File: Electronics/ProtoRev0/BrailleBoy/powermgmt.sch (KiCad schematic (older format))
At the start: 13 parts, among them J1 USB_B_Micro, J2 Battery, U4 AP2115-SOIC, U5 MCP73832-2-OT

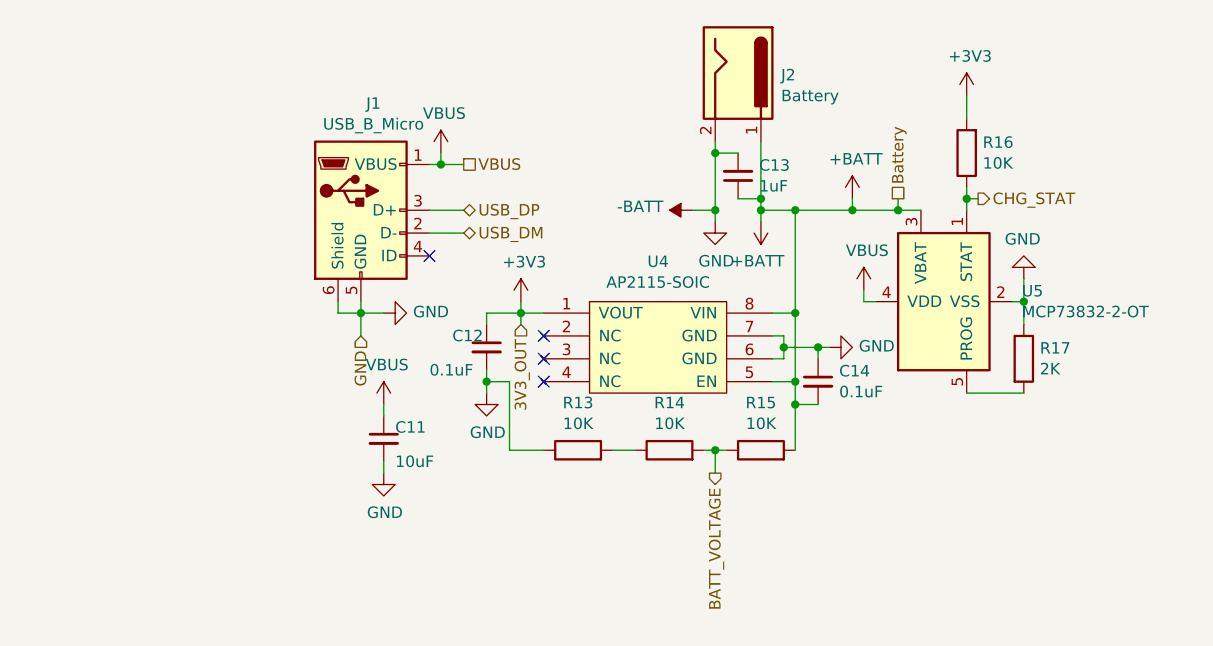
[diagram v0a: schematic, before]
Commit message: Added some annotations to make things rather professional :)
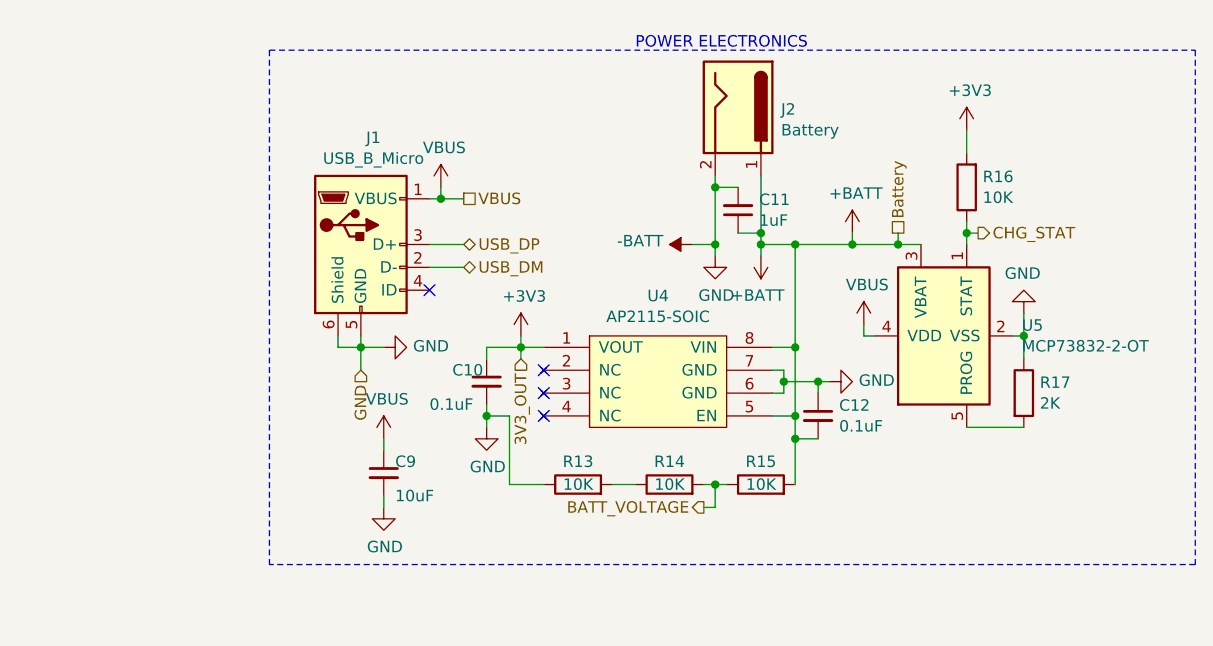
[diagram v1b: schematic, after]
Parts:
- renumbered C12 to C10, C13 to C11, C14 to C12, C11 to C9
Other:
- note added: "POWER ELECTRONICS"
- moved on the sheet: C10, C11, C12, C9, J1, J2, R13, R14, R15, R16, R17, U4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

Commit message: Made the schematic sheets a bit prettier
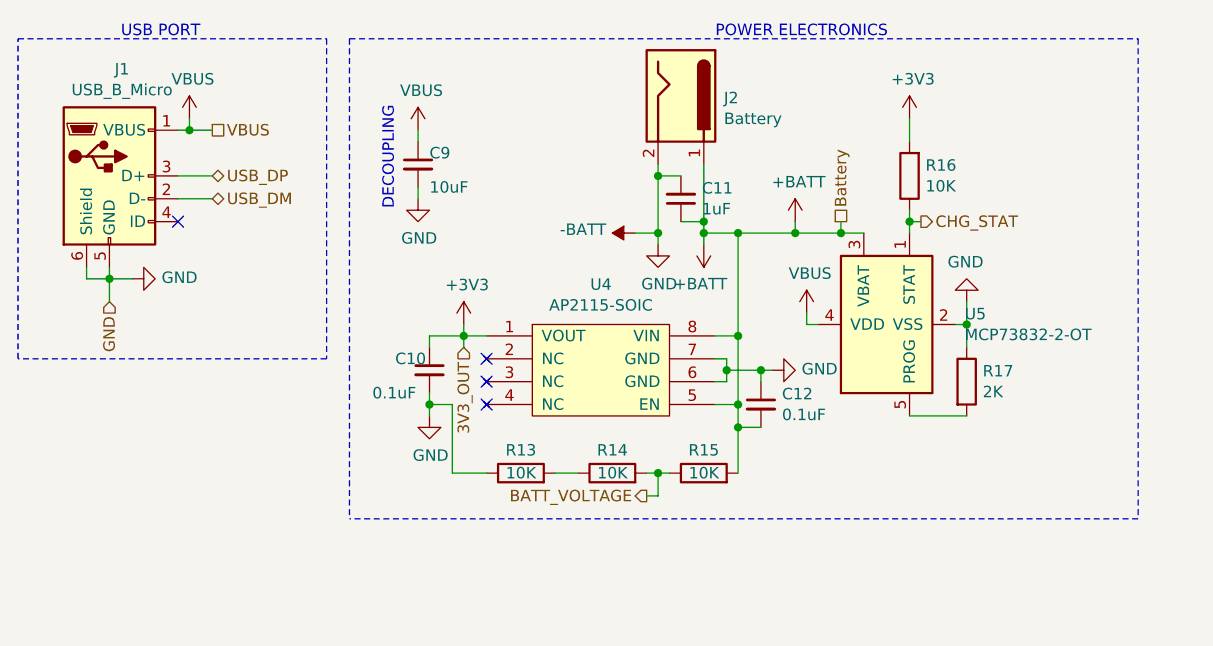
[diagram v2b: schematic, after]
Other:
- note added: "DECOUPLING"
- note added: "USB PORT"
- moved on the sheet: C10, C11, C12, C9, J1, J2, R13, R14, R15, R16, R17, U4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
